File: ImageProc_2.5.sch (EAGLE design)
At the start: 108 parts, among them IC1 XC61GC3002HR-G, IC10 AT45DB642D-CNU, IC2 MIC5335-SPYMT, IC3 MIC5335-JGYMT, IC4 DSPIC33FJ128MC706A, IC5 AT86RF233-ZU, IC6 LTC6088, IC7 DRV8833RTY, IC8 DRV8833RTY, IC9 MPU-6000, P1 BAT+, P10 MD2, P11 EXT1, P12 EXT2, P13 EXT3, P14 EXT4, P15 EXT5, P16 EXT6, P2 BAT-, P3 MA1, P4 MA2, P5 MB1, P6 MB2, P7 MC1, P8 MC2, P9 MD1

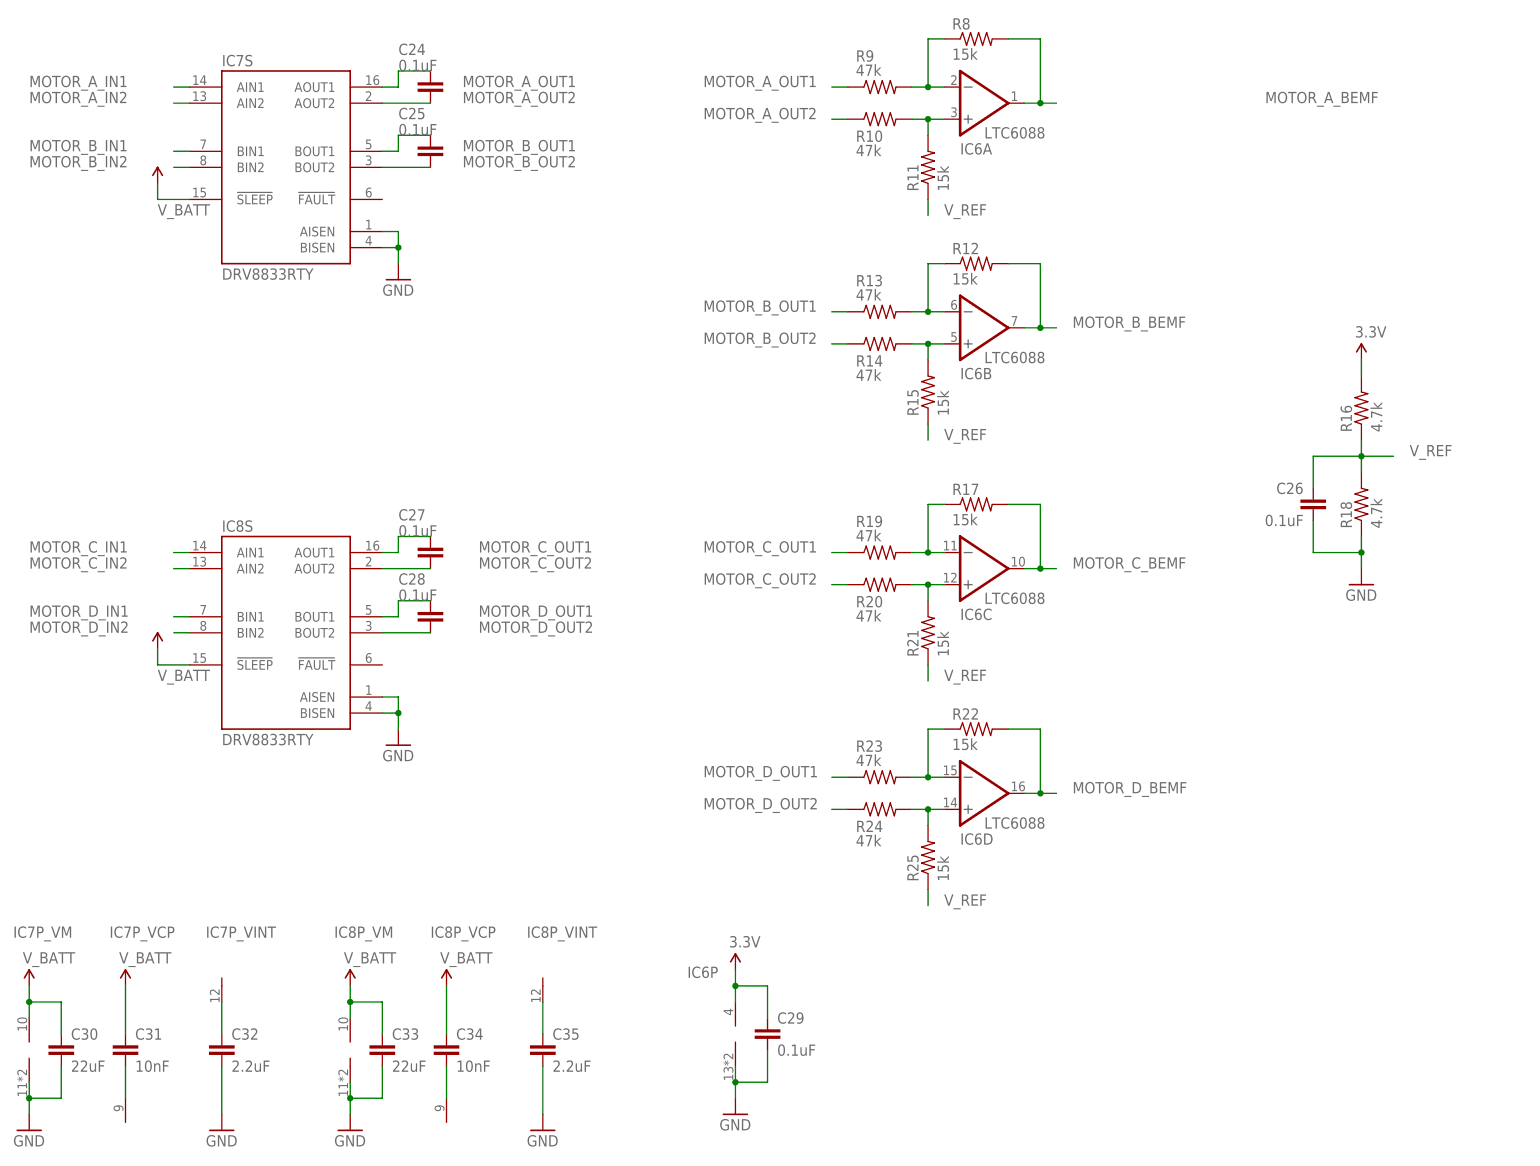
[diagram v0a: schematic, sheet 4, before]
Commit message: Commit before replace LTC6088 with LT1991
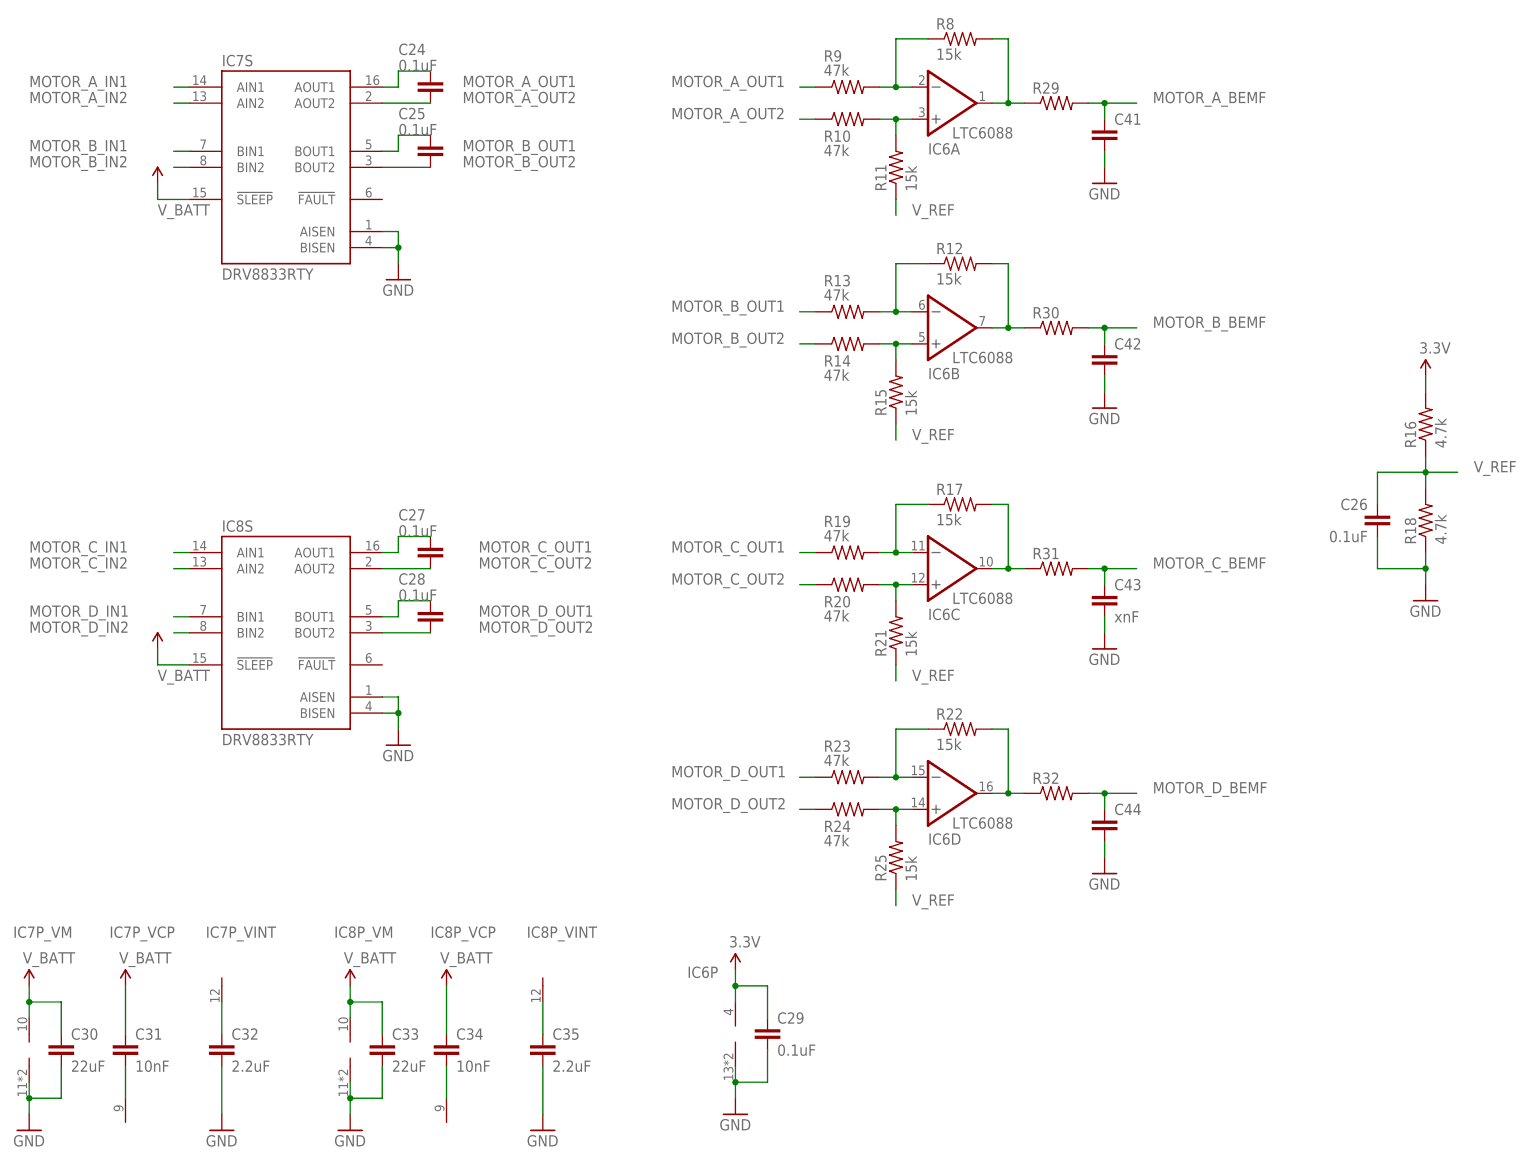
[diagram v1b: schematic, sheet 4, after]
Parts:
- added C41, C42, C44: (no value), biomimetic:CAP0402-CAP
- added C43: xnF, biomimetic:CAP0402-CAP
- added R29, R30, R31, R32: (no value), biomimetic:RESISTOR0402-RES
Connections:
- new net N$34: IC6D.OUT, R22.2, R32.1
- new net N$35: IC6C.OUT, R17.2, R31.1
- new net N$36: IC6A.OUT, R29.1, R8.2
- new net N$37: IC6B.OUT, R12.2, R30.1
- net GND: now also C41.2, C42.2, C43.2, C44.2
- net MOTOR_A_BEMF: now also C41.1, R29.2; no longer IC6A.OUT, R8.2
- net MOTOR_B_BEMF: now also C42.1, R30.2; no longer IC6B.OUT, R12.2
- net MOTOR_C_BEMF: now also C43.1, R31.2; no longer IC6C.OUT, R17.2
- net MOTOR_D_BEMF: now also C44.1, R32.2; no longer IC6D.OUT, R22.2
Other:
- moved on the sheet: C26, IC6A, IC6B, IC6C, IC6D, R10, R11, R12, R13, R14, R15, R16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
